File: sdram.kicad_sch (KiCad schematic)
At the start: 2 parts, among them U1 ECP5U_12_CABGA256, U10 W9825G6KH-6

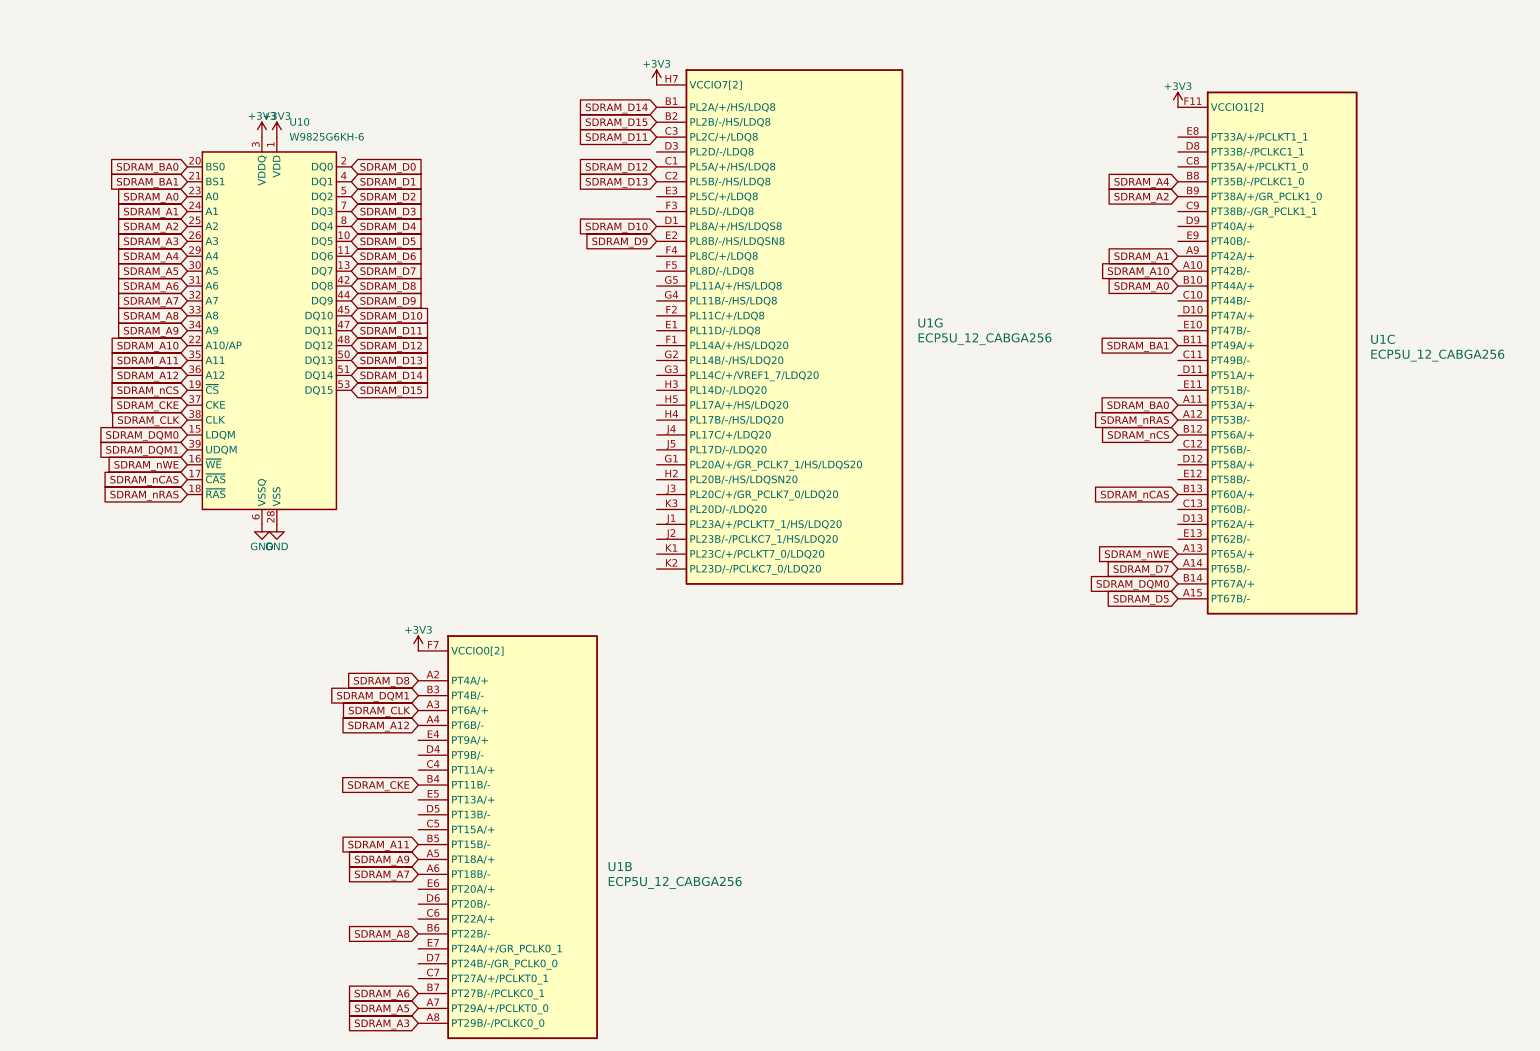
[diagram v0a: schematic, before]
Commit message: Stash
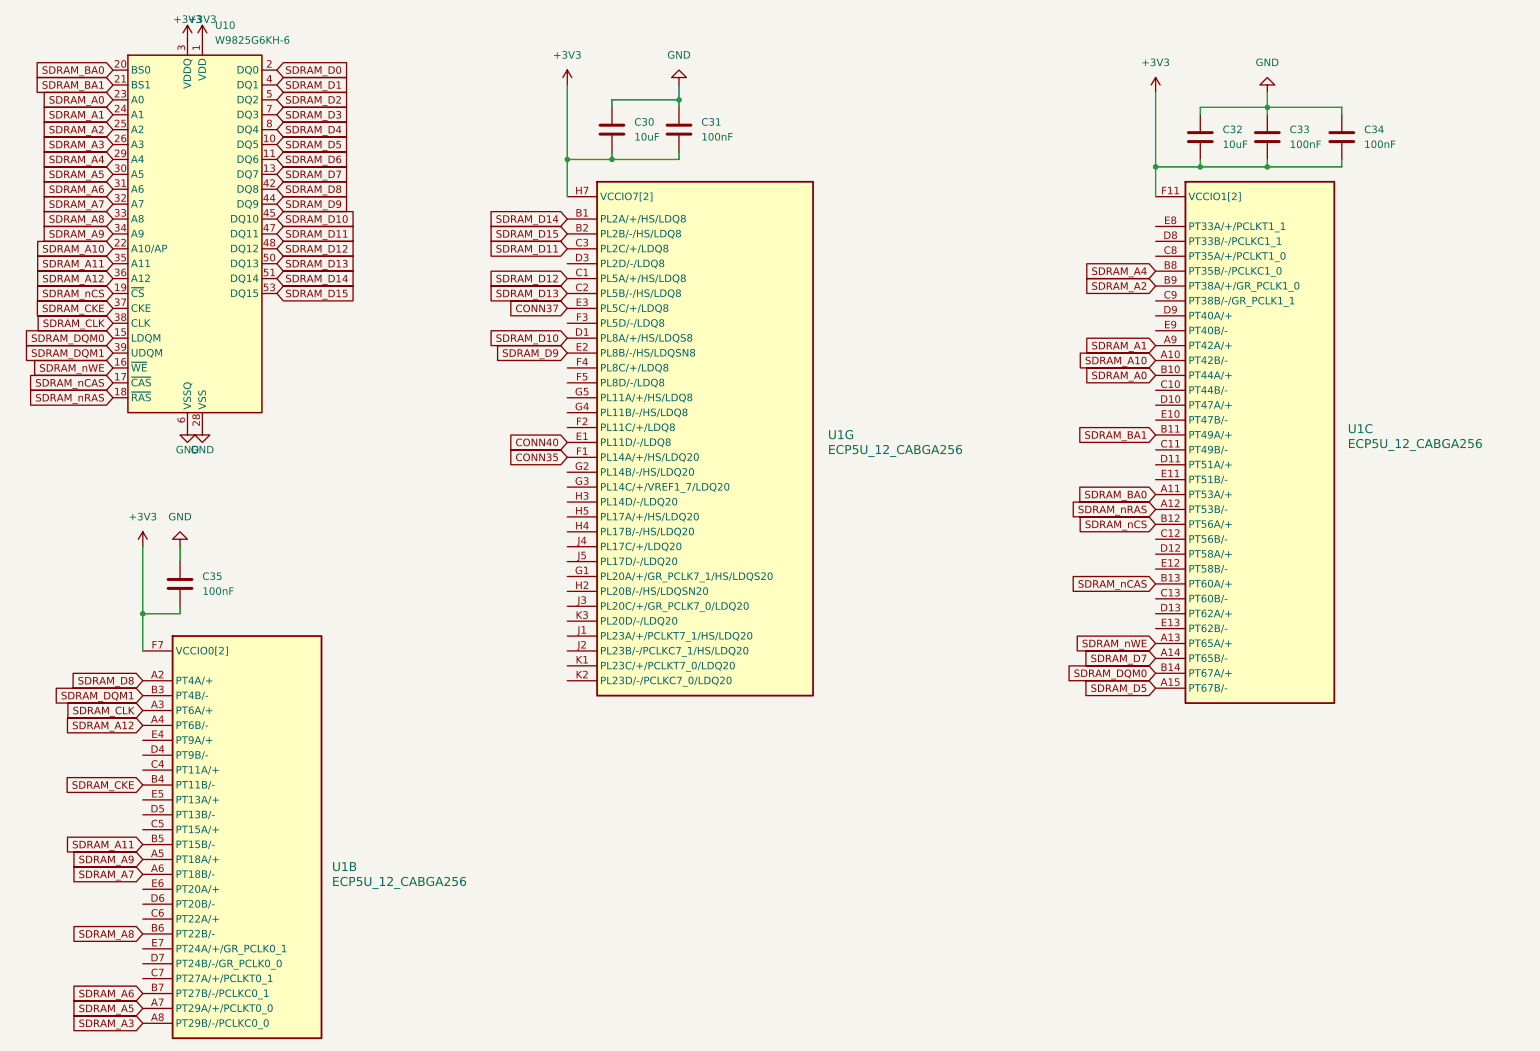
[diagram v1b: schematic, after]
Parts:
- added C30, C32: 10uF, Capacitor_SMD:C_0603_1608Metric, symbol Device:C
- added C31, C33, C34, C35: 100nF, Capacitor_SMD:C_0402_1005Metric, symbol Device:C
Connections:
- net +3V3: now also C30.2, C31.2, C32.2, C33.2, C34.2, C35.2
- net GND: now also C30.1, C31.1, C32.1, C33.1, C34.1, C35.1
- net CONN40: now reaches U1.E1 (PL11D/-/LDQ8)
- net CONN37: now reaches U1.E3 (PL5C/+/LDQ8)
- net CONN35: now reaches U1.F1 (PL14A/+/HS/LDQ20)
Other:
- moved on the sheet: U10, U1B, U1C, U1G
